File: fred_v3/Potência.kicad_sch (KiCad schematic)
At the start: 0 parts

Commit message: Add files via upload
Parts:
- added D20, D21: 1N4728A, Diode_THT:D_DO-41_SOD81_P10.16mm_Horizontal, symbol Device:D_Zener
- added J17: MOTOR1_F, TerminalBlock_Phoenix:TerminalBlock_Phoenix_MKDS-3-2-5.08_1x02_P5.08mm_Horizontal, symbol Connector_Generic:Conn_01x02
- added J18: MOTOR2_F, TerminalBlock_Phoenix:TerminalBlock_Phoenix_MKDS-3-2-5.08_1x02_P5.08mm_Horizontal, symbol Connector_Generic:Conn_01x02
- added J19: MOTOR1_B, TerminalBlock_Phoenix:TerminalBlock_Phoenix_MKDS-3-2-5.08_1x02_P5.08mm_Horizontal, symbol Connector_Generic:Conn_01x02
- added J20: MOTOR2_B, TerminalBlock_Phoenix:TerminalBlock_Phoenix_MKDS-3-2-5.08_1x02_P5.08mm_Horizontal, symbol Connector_Generic:Conn_01x02
- added J28 (x2): Conn_02x04_Odd_Even, Connector_IDC:IDC-Header_2x04_P2.54mm_Vertical, symbol Connector_Generic:Conn_02x04_Odd_Even
- added R38, R71: 8k, Resistor_SMD:R_0603_1608Metric_Pad0.98x0.95mm_HandSolder, symbol Device:R
- added R39, R40: 2k, Resistor_SMD:R_0603_1608Metric_Pad0.98x0.95mm_HandSolder, symbol Device:R
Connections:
- new net 3,3V_Back: D20.1 (K), R38.1, R39.2
- new net 3,3V_Front: D21.1 (K), R40.2, R71.1
- new net 5V: R39.1, R40.1
- new net Current_Sense1: J28.2 (Pin_2)
- new net Current_Sense2: J28.4 (Pin_4)
- new net Current_Sense3: J28.2 (Pin_2)
- new net Current_Sense4: J28.4 (Pin_4)
- new net GND: D20.2 (A), D21.2 (A), R38.2, R71.2
- new net INA_M1_BACK: J28.1 (Pin_1)
- new net INA_M1_FRONT: J28.1 (Pin_1)
- new net INA_M2_BACK: J28.7 (Pin_7)
- new net INA_M2_FRONT: J28.7 (Pin_7)
- new net INB_M1_BACK: J28.3 (Pin_3)
- new net INB_M1_FRONT: J28.3 (Pin_3)
- new net INB_M2_BACK: J28.6 (Pin_6)
- new net INB_M2_FRONT: J28.6 (Pin_6)
- new net Motors_Back/OUTA_M2_BACK: J20.2 (Pin_2)
- new net Motors_Back/OUTB_M1_BACK: J19.2 (Pin_2)
- new net Motors_Front/OUTB_M1_FRONT: J17.2 (Pin_2)
- new net Motors_Front/OUTB_M2_FRONT: J18.2 (Pin_2)
- new net PWM_M1_BACK: J28.5 (Pin_5)
- new net PWM_M1_FRONT: J28.5 (Pin_5)
- new net PWM_M2_BACK: J28.8 (Pin_8)
- new net PWM_M2_FRONT: J28.8 (Pin_8)
- new net Sensor_Corrente1/IP-: J17.1 (Pin_1)
- new net Sensor_Corrente2/IP-: J18.1 (Pin_1)
- new net Sensor_Corrente3/IP-: J19.1 (Pin_1)
- new net Sensor_Corrente4/IP-: J20.1 (Pin_1)
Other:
- added sheet Isolamento1 (Isolamento.kicad_sch)
- added sheet Isolamento2 (Isolamento.kicad_sch)
- added sheet Motors_Back (Motors_Back.kicad_sch)
- added sheet Motors_Front (Motors_Front.kicad_sch)
- added sheet Sensor_Corrente1 (Sensor_Corrente.kicad_sch)
- added sheet Sensor_Corrente2 (Sensor_Corrente.kicad_sch)
- added sheet Sensor_Corrente3 (Sensor_Corrente.kicad_sch)
- added sheet Sensor_Corrente4 (Sensor_Corrente.kicad_sch)

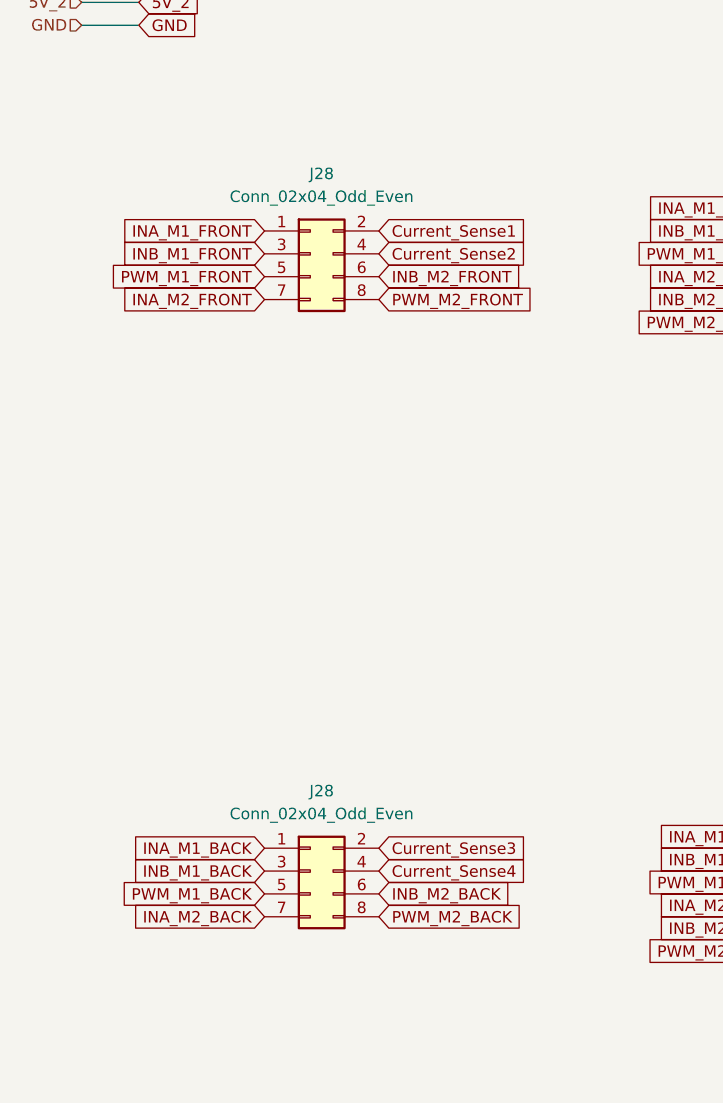
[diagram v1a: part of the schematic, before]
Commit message: Add files via upload
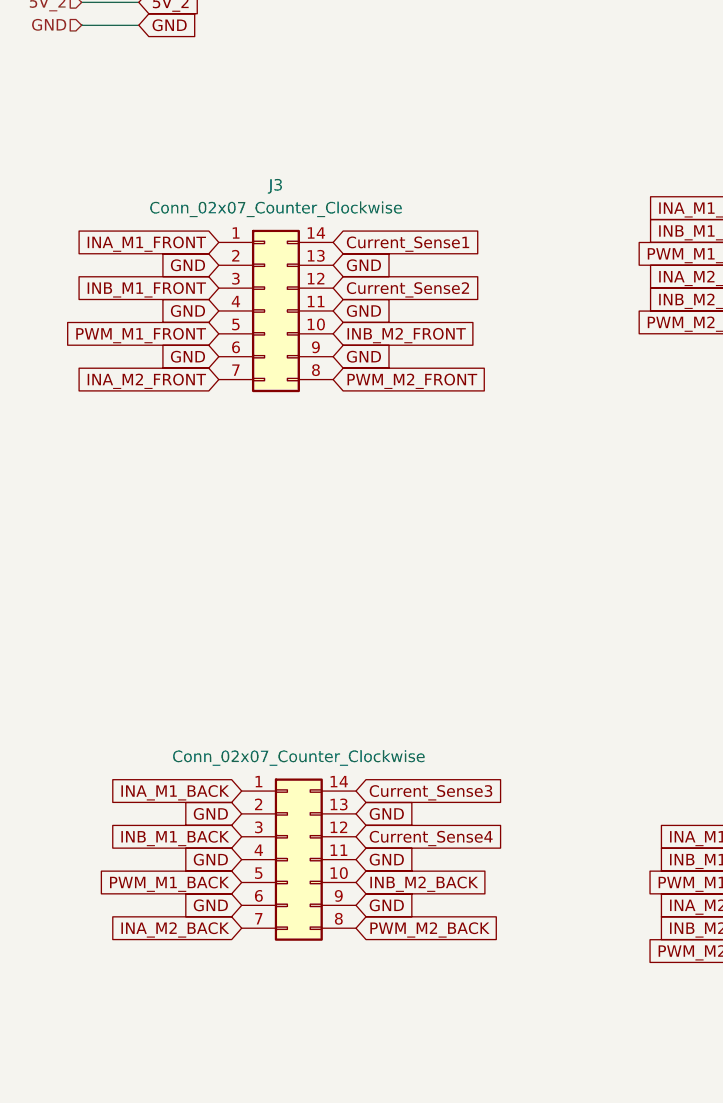
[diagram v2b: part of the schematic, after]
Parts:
- removed J28 (x2): Conn_02x04_Odd_Even, Connector_IDC:IDC-Header_2x04_P2.54mm_Vertical, symbol Connector_Generic:Conn_02x04_Odd_Even
- added J2, J3: Conn_02x07_Counter_Clockwise, Connector_IDC:IDC-Header_2x07_P2.54mm_Vertical, symbol Connector_Generic:Conn_02x07_Counter_Clockwise
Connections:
- net Current_Sense1: now also J3.14 (Pin_14)
- net Current_Sense2: now also J3.12 (Pin_12)
- net Current_Sense3: now also J2.14 (Pin_14)
- net Current_Sense4: now also J2.12 (Pin_12)
- net GND: now also J2.11 (Pin_11), J2.13 (Pin_13), J2.2 (Pin_2), J2.4 (Pin_4), J2.6 (Pin_6), J2.9 (Pin_9), J3.11 (Pin_11), J3.13 (Pin_13), J3.2 (Pin_2), J3.4 (Pin_4), J3.6 (Pin_6), J3.9 (Pin_9)
- net INA_M1_BACK: now also J2.1 (Pin_1)
- net INA_M1_FRONT: now also J3.1 (Pin_1)
- net INA_M2_BACK: now also J2.7 (Pin_7)
- net INA_M2_FRONT: now also J3.7 (Pin_7)
- net INB_M1_BACK: now also J2.3 (Pin_3)
- net INB_M1_FRONT: now also J3.3 (Pin_3)
- net INB_M2_BACK: now also J2.10 (Pin_10)
- net INB_M2_FRONT: now also J3.10 (Pin_10)
- net PWM_M1_BACK: now also J2.5 (Pin_5)
- net PWM_M1_FRONT: now also J3.5 (Pin_5)
- net PWM_M2_BACK: now also J2.8 (Pin_8)
- net PWM_M2_FRONT: now also J3.8 (Pin_8)

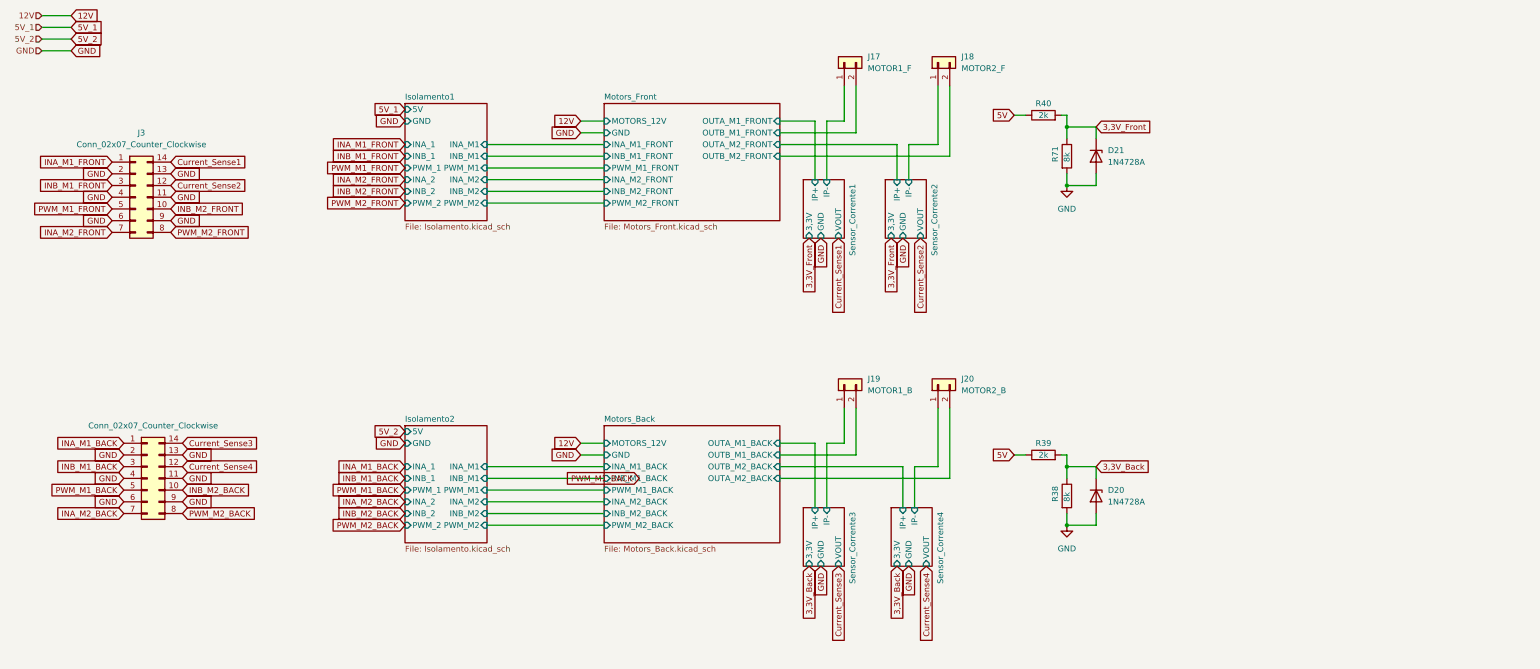
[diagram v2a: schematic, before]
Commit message: Add files via upload
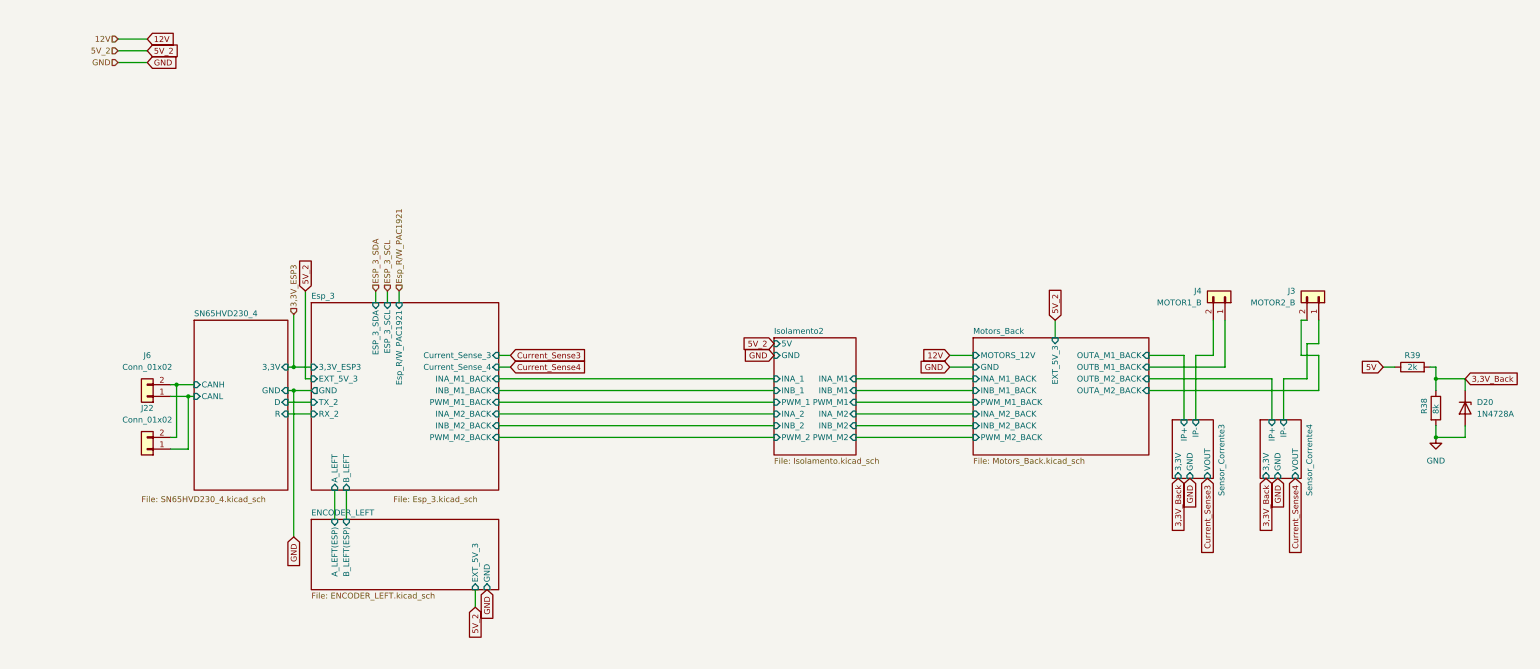
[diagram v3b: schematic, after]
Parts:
- removed D21: 1N4728A, Diode_THT:D_DO-41_SOD81_P10.16mm_Horizontal, symbol Device:D_Zener
- removed J17: MOTOR1_F, TerminalBlock_Phoenix:TerminalBlock_Phoenix_MKDS-3-2-5.08_1x02_P5.08mm_Horizontal, symbol Connector_Generic:Conn_01x02
- removed J18: MOTOR2_F, TerminalBlock_Phoenix:TerminalBlock_Phoenix_MKDS-3-2-5.08_1x02_P5.08mm_Horizontal, symbol Connector_Generic:Conn_01x02
- removed J19: MOTOR1_B, TerminalBlock_Phoenix:TerminalBlock_Phoenix_MKDS-3-2-5.08_1x02_P5.08mm_Horizontal, symbol Connector_Generic:Conn_01x02
- removed J2, J3: Conn_02x07_Counter_Clockwise, Connector_IDC:IDC-Header_2x07_P2.54mm_Vertical, symbol Connector_Generic:Conn_02x07_Counter_Clockwise
- removed J20: MOTOR2_B, TerminalBlock_Phoenix:TerminalBlock_Phoenix_MKDS-3-2-5.08_1x02_P5.08mm_Horizontal, symbol Connector_Generic:Conn_01x02
- removed R40: 2k, Resistor_SMD:R_0603_1608Metric_Pad0.98x0.95mm_HandSolder, symbol Device:R
- removed R71: 8k, Resistor_SMD:R_0603_1608Metric_Pad0.98x0.95mm_HandSolder, symbol Device:R
- added J22, J6: Conn_01x02, TerminalBlock_Phoenix:TerminalBlock_Phoenix_MKDS-3-2-5.08_1x02_P5.08mm_Horizontal, symbol Connector_Generic:Conn_01x02
- added J3: MOTOR2_B, TerminalBlock_Phoenix:TerminalBlock_Phoenix_MKDS-3-2-5.08_1x02_P5.08mm_Horizontal, symbol Connector_Generic:Conn_01x02
- added J4: MOTOR1_B, TerminalBlock_Phoenix:TerminalBlock_Phoenix_MKDS-3-2-5.08_1x02_P5.08mm_Horizontal, symbol Connector_Generic:Conn_01x02
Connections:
- net Motors_Back/OUTA_M2_BACK: now also J3.2 (Pin_2)
- net Motors_Back/OUTB_M1_BACK: now also J4.1 (Pin_1)
- net Sensor_Corrente3/IP-: now also J4.2 (Pin_2)
- net Sensor_Corrente4/IP-: now also J3.1 (Pin_1)
- new net SN65HVD230_4/CANH: J22.2 (Pin_2), J6.2 (Pin_2)
- new net SN65HVD230_4/CANL: J22.1 (Pin_1), J6.1 (Pin_1)
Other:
- removed sheet Isolamento1
- removed sheet Motors_Front
- removed sheet Sensor_Corrente1
- removed sheet Sensor_Corrente2
- added sheet ENCODER_LEFT (ENCODER_LEFT.kicad_sch)
- added sheet Esp_3 (Esp_3.kicad_sch)
- added sheet SN65HVD230_4 (SN65HVD230_4.kicad_sch)
- sheet Motors_Back ports: added EXT_5V_3; removed none
- moved on the sheet: D20, R38, R39
